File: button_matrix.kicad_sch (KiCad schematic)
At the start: 142 parts

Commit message: add zefir to da mix
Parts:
- MX1, MX10, MX11, MX12, MX13, MX14, MX15, MX16, MX17, MX18, MX19, MX2, MX20, MX21, MX22, MX23, MX24, MX25, MX26, MX27, MX28, MX29, MX3, MX30, MX31, MX32, MX33, MX34, MX35, MX36, MX37, MX38, MX39, MX4, MX40, MX41, MX42, MX43, MX44, MX45, MX46, MX47, MX48, MX49, MX5, MX50, MX51, MX52, MX53, MX54, MX55, MX56, MX57, MX58, MX59, MX6, MX60, MX61, MX62, MX63, MX64, MX7, MX8, MX9: footprint Arcade_Switch:MM9-3-AU-withbutton -> Arcade_Switch:MM9-3-AU-withbutton-notxt

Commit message: update shit
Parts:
- S1, S2, S3, S4, S5, S6, S7: footprint TS11-674-120-BK-100-RA-D:SW_TS11-674-120-BK-100-RA-D -> TS11-674-120-BK-100-RA-D:SW_TS11-674-120-BK-100-RA-D-notxt
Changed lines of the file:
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@@
 			)
 		)
-		(property "Footprint" "TS11-674-120-BK-100-RA-D:SW_TS11-674-120-BK-100-RA-D"
+		(property "Footprint" "TS11-674-120-BK-100-RA-D:SW_TS11-674-120-BK-100-RA-D-notxt"
 			(at 187.96 116.84 0)
 			(effects
@@
 			)
 		)
-		(property "Footprint" "TS11-674-120-BK-100-RA-D:SW_TS11-674-120-BK-100-RA-D"
+		(property "Footprint" "TS11-674-120-BK-100-RA-D:SW_TS11-674-120-BK-100-RA-D-notxt"
 			(at 232.41 132.08 0)
 			(effects
@@
 			)
 		)
-		(property "Footprint" "TS11-674-120-BK-100-RA-D:SW_TS11-674-120-BK-100-RA-D"
+		(property "Footprint" "TS11-674-120-BK-100-RA-D:SW_TS11-674-120-BK-100-RA-D-notxt"
 			(at 187.96 138.43 0)
 			(effects
@@
 			)
 		)
-		(property "Footprint" "TS11-674-120-BK-100-RA-D:SW_TS11-674-120-BK-100-RA-D"
+		(property "Footprint" "TS11-674-120-BK-100-RA-D:SW_TS11-674-120-BK-100-RA-D-notxt"
 			(at 184.15 35.56 0)
 			(effects
@@
 			)
 		)
-		(property "Footprint" "TS11-674-120-BK-100-RA-D:SW_TS11-674-120-BK-100-RA-D"
+		(property "Footprint" "TS11-674-120-BK-100-RA-D:SW_TS11-674-120-BK-100-RA-D-notxt"
 			(at 187.96 95.25 0)
 			(effects
@@
 			)
 		)
-		(property "Footprint" "TS11-674-120-BK-100-RA-D:SW_TS11-674-120-BK-100-RA-D"
+		(property "Footprint" "TS11-674-120-BK-100-RA-D:SW_TS11-674-120-BK-100-RA-D-notxt"
 			(at 187.96 78.74 0)
 			(effects
@@
 			)
 		)
-		(property "Footprint" "TS11-674-120-BK-100-RA-D:SW_TS11-674-120-BK-100-RA-D"
+		(property "Footprint" "TS11-674-120-BK-100-RA-D:SW_TS11-674-120-BK-100-RA-D-notxt"
 			(at 187.96 57.15 0)
 			(effects

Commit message: update
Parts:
- D1, D10, D11, D12, D13, D14, D15, D16, D17, D18, D19, D193, D194, D195, D196, D197, D198, D199, D2, D20, D21, D22, D23, D24, D25, D26, D27, D28, D29, D3, D30, D31, D32, D33, D34, D35, D36, D37, D38, D39, D4, D40, D41, D42, D43, D44, D45, D46, D47, D48, D49, D5, D50, D51, D52, D53, D54, D55, D56, D57, D58, D59, D6, D60, D61, D62, D63, D64, D7, D8, D9: footprint Diode_SMD:D_0603_1608Metric-notxt -> Diode_SMD:D_SOD-123-notxt

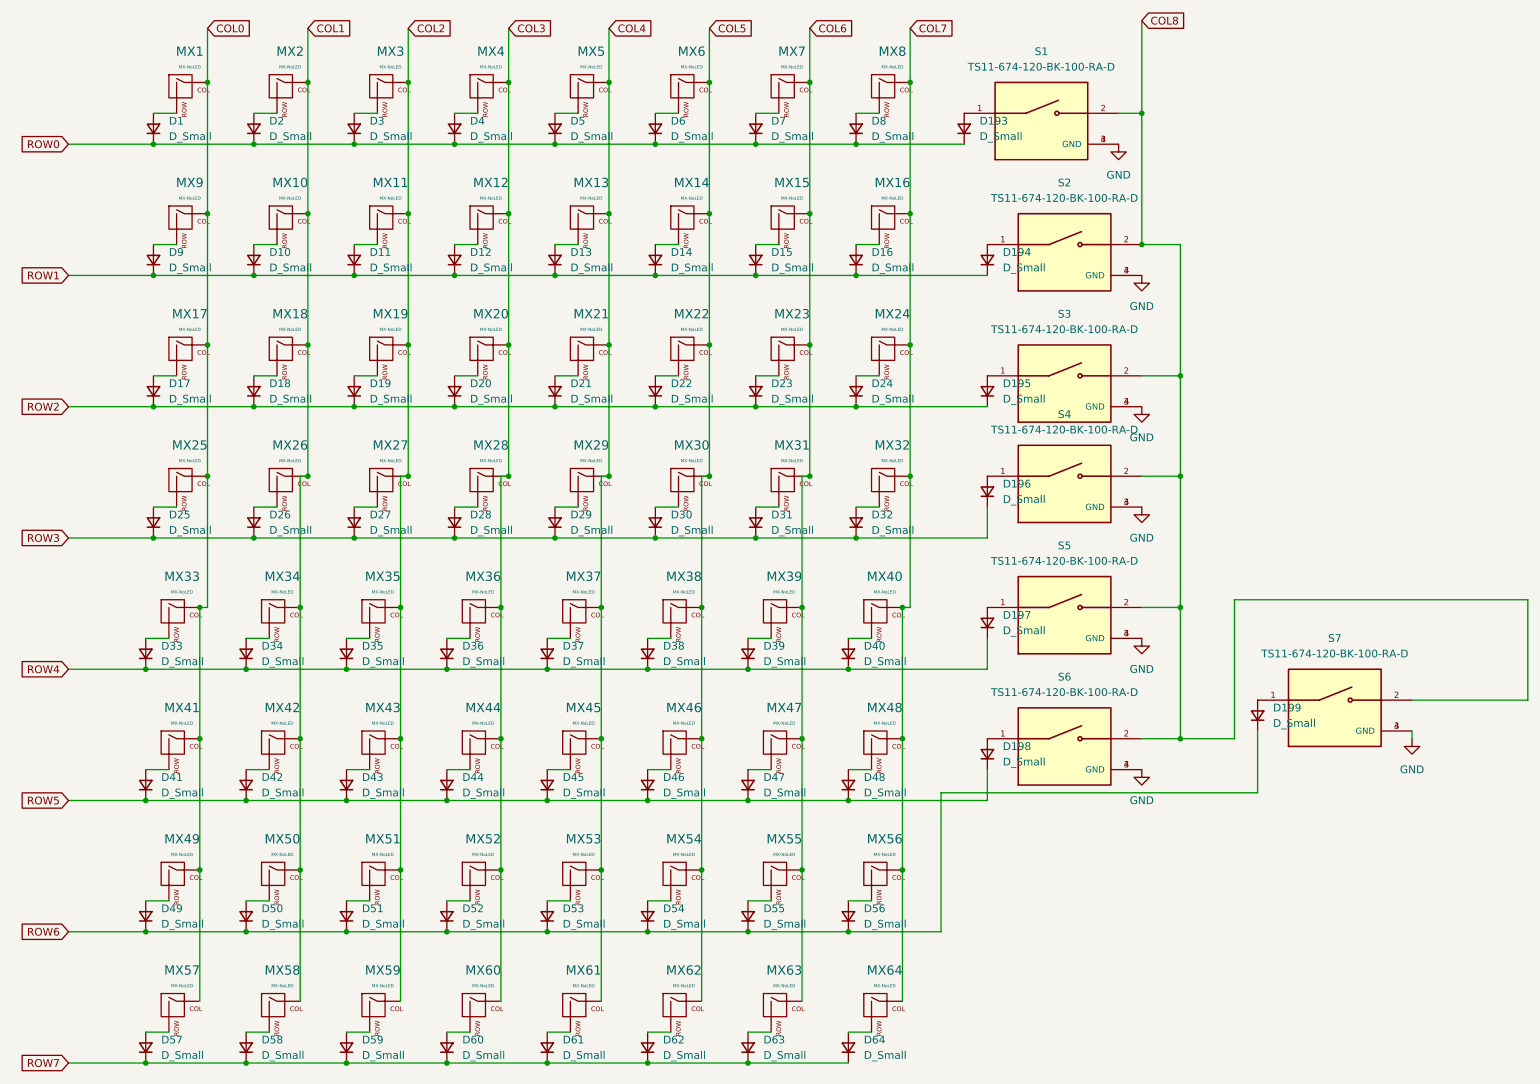
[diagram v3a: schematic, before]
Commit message: yeah have some updates my g
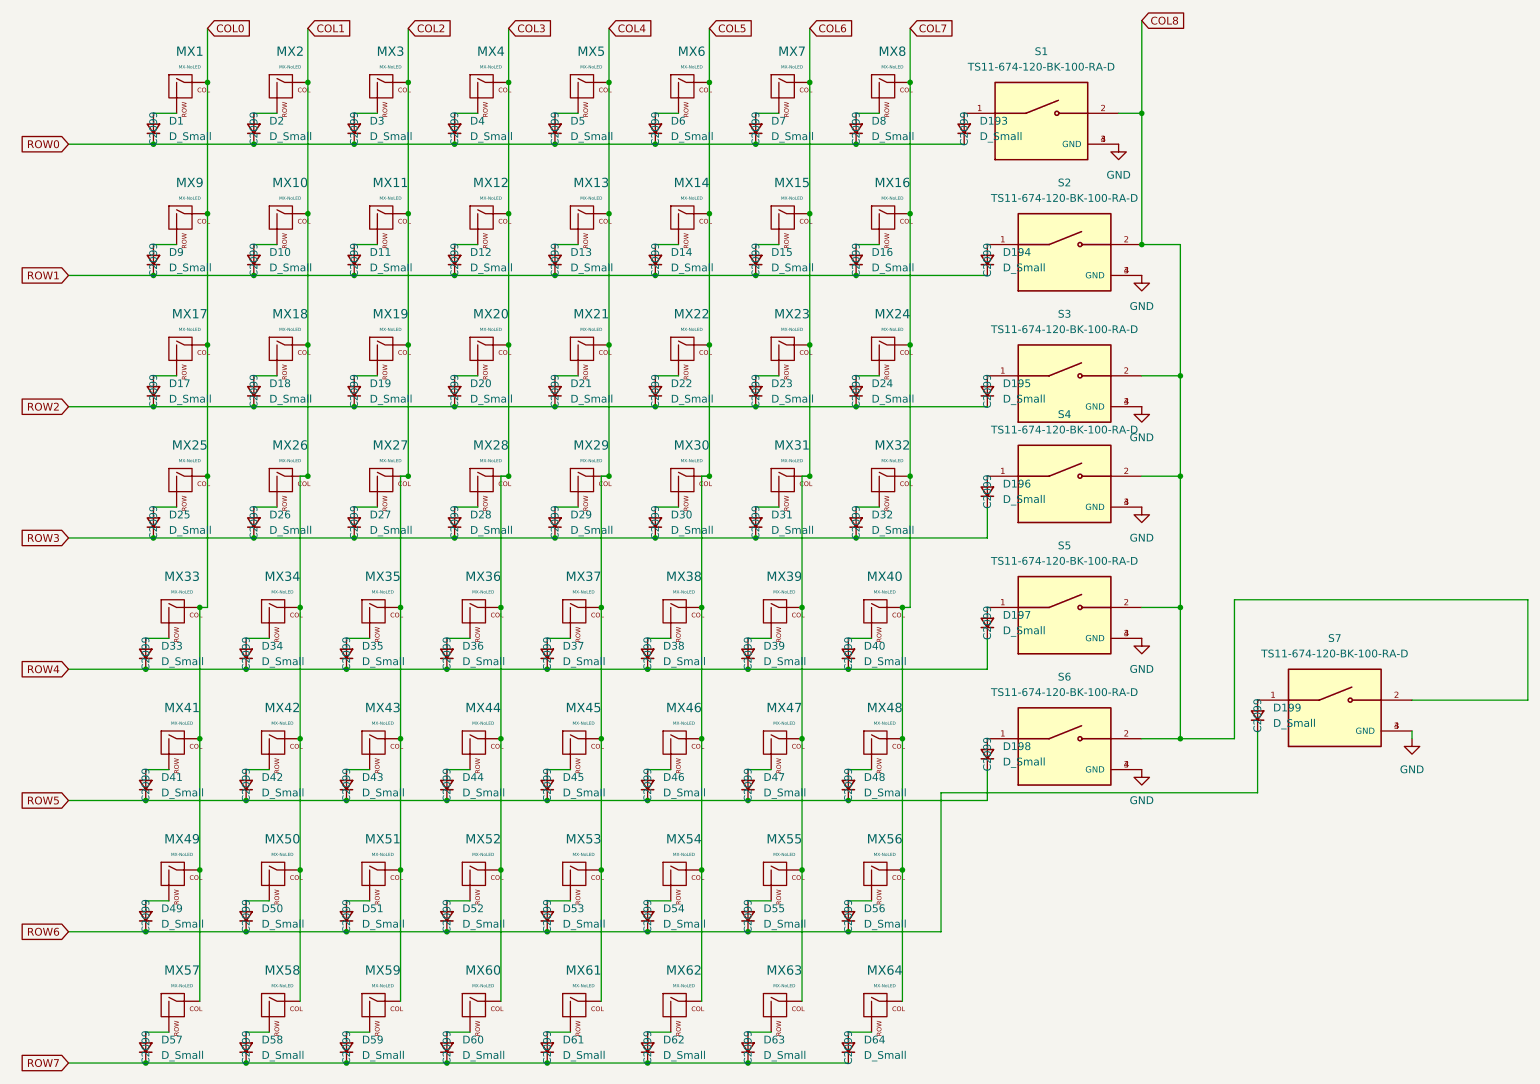
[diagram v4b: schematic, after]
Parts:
- D1, D10, D11, D12, D13, D14, D15, D16, D17, D18, D19, D193, D194, D195, D196, D197, D198, D199, D2, D20, D21, D22, D23, D24, D25, D26, D27, D28, D29, D3, D30, D31, D32, D33, D34, D35, D36, D37, D38, D39, D4, D40, D41, D42, D43, D44, D45, D46, D47, D48, D49, D5, D50, D51, D52, D53, D54, D55, D56, D57, D58, D59, D6, D60, D61, D62, D63, D64, D7, D8, D9: JLCPCB Part (none) -> C2099
- MX1, MX10, MX11, MX12, MX13, MX14, MX15, MX16, MX17, MX18, MX19, MX2, MX20, MX21, MX22, MX23, MX24, MX25, MX26, MX27, MX28, MX29, MX3, MX30, MX31, MX32, MX33, MX34, MX35, MX36, MX37, MX38, MX39, MX4, MX40, MX41, MX42, MX43, MX44, MX45, MX46, MX47, MX48, MX49, MX5, MX50, MX51, MX52, MX53, MX54, MX55, MX56, MX57, MX58, MX59, MX6, MX60, MX61, MX62, MX63, MX64, MX7, MX8, MX9, S1, S2, S3, S4, S5, S6, S7: now left out of the parts list
